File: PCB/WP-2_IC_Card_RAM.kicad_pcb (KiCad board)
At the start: 2 copper layers, 45 x 54 mm, 11 parts, among them J1 Conn_01x38_Female, U1 SRAM 128Kx8 5v Parallel, U2 SRAM 128Kx8 5v Parallel

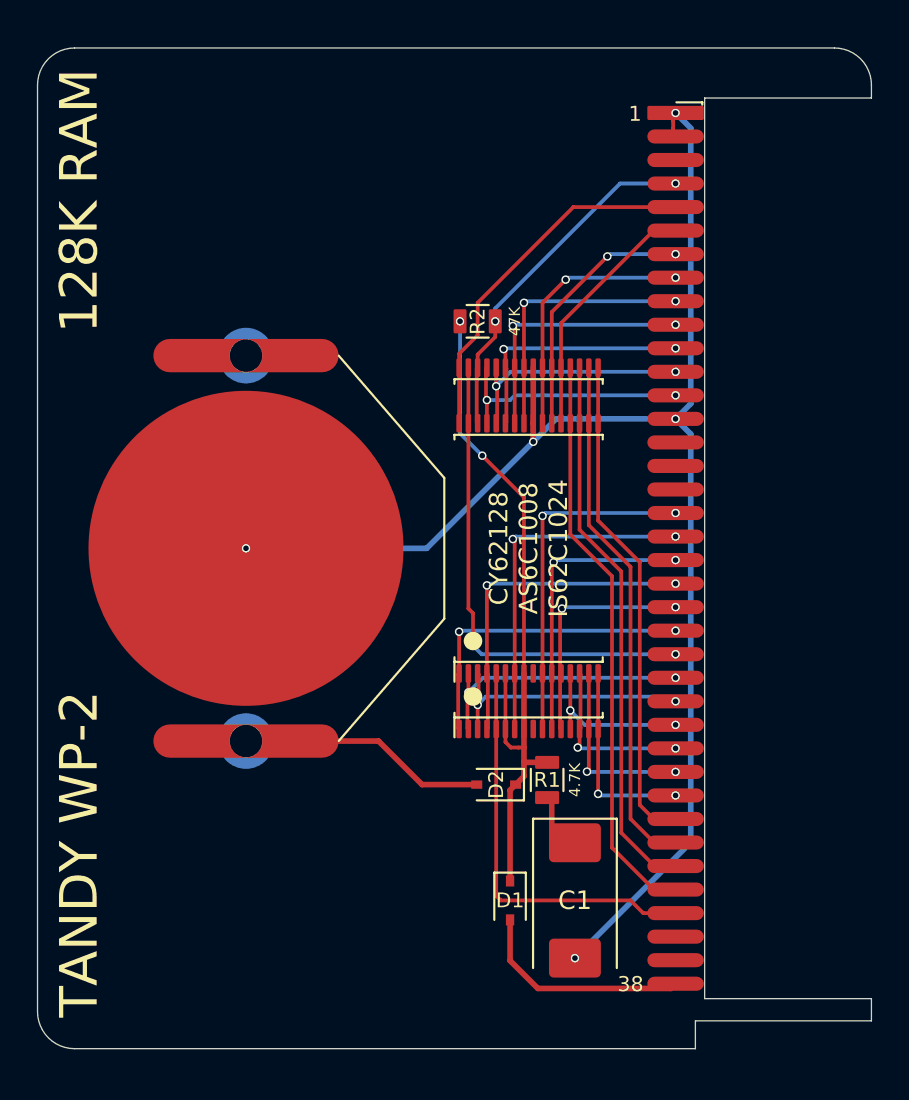
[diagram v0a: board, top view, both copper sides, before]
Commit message: readme
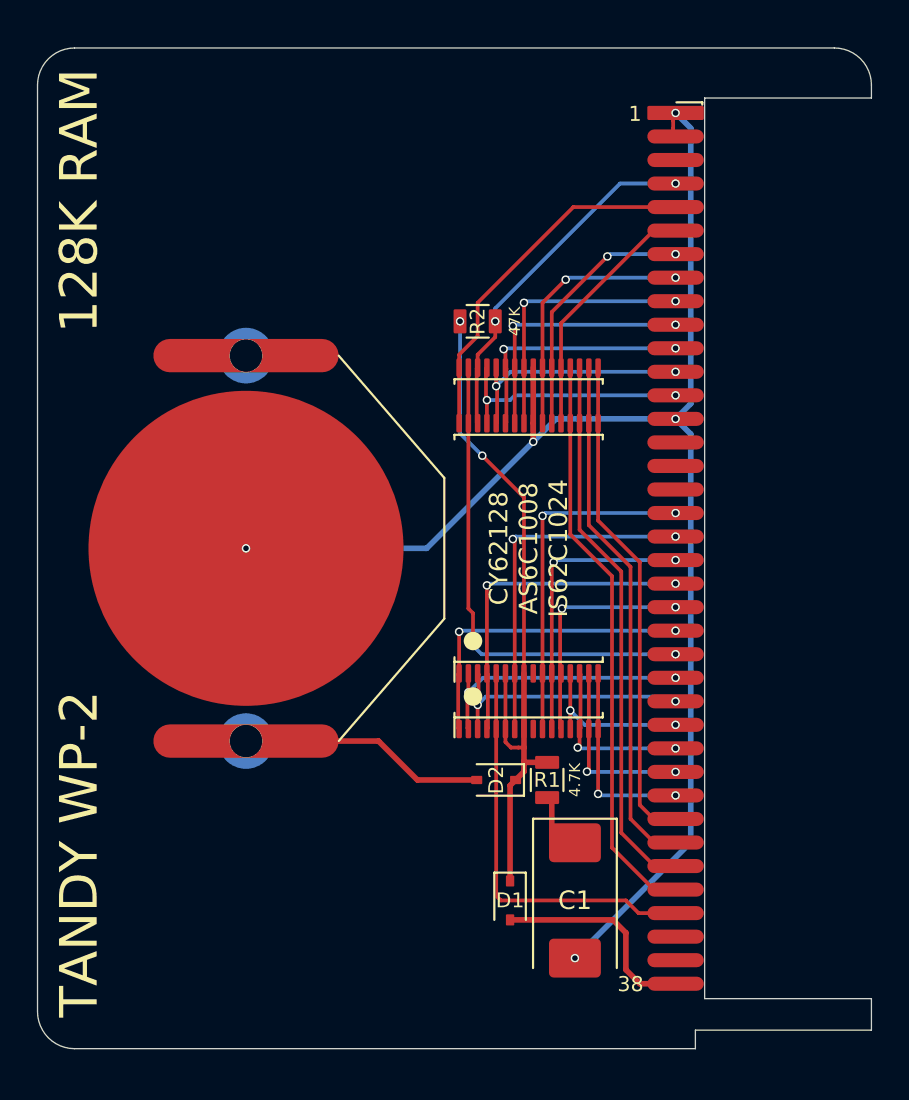
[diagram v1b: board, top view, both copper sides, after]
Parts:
- moved D2 0.25 mm to (147.5, 112.2)
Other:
- outline, holes or cut-outs redrawn
